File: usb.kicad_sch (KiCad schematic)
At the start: 4 parts, among them J2 SHOU HAN TYPE-C 16PIN 2MD(073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

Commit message: #1 Use new central library KiCad-Lib
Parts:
- J2: footprint Project_Library:SHOU HAN TYPE-C 16PIN 2MD(073) (C2765186) -> #Connector:SHOU HAN TYPE-C 16PIN 2MD(073); symbol Project_Library:SHOU HAN TYPE-C 16PIN 2MD(073) (C2765186) -> #Connector:SHOU HAN TYPE-C 16PIN 2MD(073)
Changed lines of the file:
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@@
     (effects (font (size 1 1)) (justify right))
   )
-  (symbol (lib_id "Project_Library:SHOU HAN TYPE-C 16PIN 2MD(073) (C2765186)") (at 117.475 50.165 0) (mirror y) (unit 1)
+  (symbol (lib_id "#Connector:SHOU HAN TYPE-C 16PIN 2MD(073)") (at 117.475 50.165 0) (mirror y) (unit 1)
     (in_bom yes) (on_board yes) (dnp no)
     (property "Reference" "J2" (at 128.905 48.895 0)
@@
       (effects (font (size 1.27 1.27)) (justify right))
     )
-    (property "Footprint" "Project_Library:SHOU HAN TYPE-C 16PIN 2MD(073) (C2765186)" (at 116.967 82.677 0)
+    (property "Footprint" "#Connector:SHOU HAN TYPE-C 16PIN 2MD(073)" (at 116.967 82.677 0)
       (effects (font (size 1.27 1.27)) hide)
     )
-    (property "Datasheet" "https://datasheet.lcsc.com/lcsc/2111231930_SHOU-HAN-TYPE-C-16PIN-2MD-073_C2765186.pdf" (at 118.999 80.391 0)
+    (property "Datasheet" "${KIPRJMOD}/KiCad-Lib/#Connector.doc/SHOU HAN TYPE-C 16PIN 2MD(073).pdf" (at 118.999 80.391 0)
       (effects (font (size 1.27 1.27)) hide)
     )
@@
       (effects (font (size 1.27 1.27)) hide)
     )
-    (property "JLCPCB Part #" "C2765186" (at 117.475 85.725 0)
+    (property "JLCPCB Part #" "C2765186" (at 117.475 85.725 0) (show_name)
       (effects (font (size 1.27 1.27)) hide)
     )
-    (property "isBasicPart" "NO" (at 117.475 95.885 0)
+    (property "isBasicPart" "NO" (at 117.475 95.885 0) (show_name)
       (effects (font (size 1.27 1.27)) hide)
     )

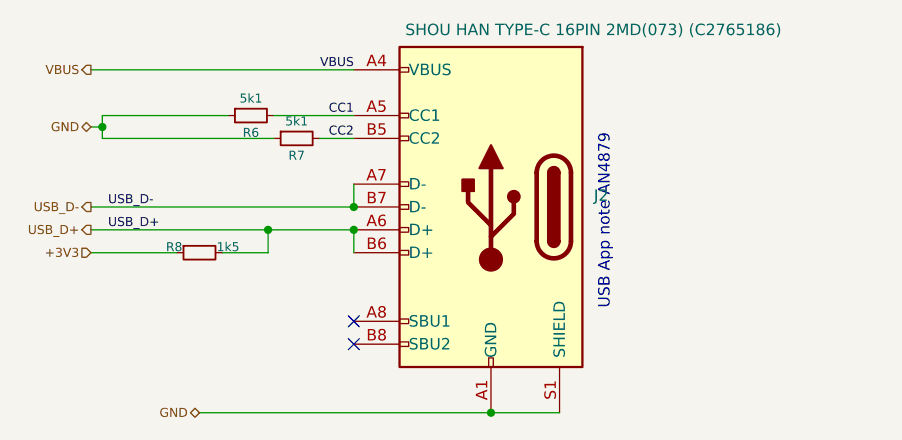
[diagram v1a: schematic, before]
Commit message: WIP
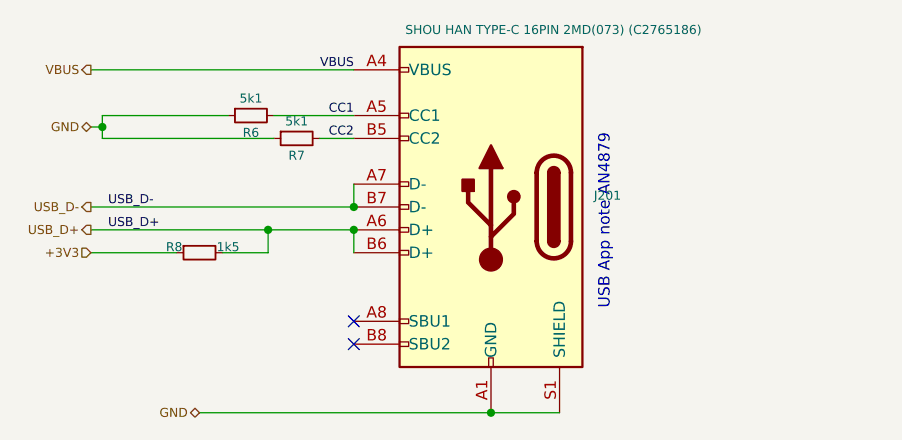
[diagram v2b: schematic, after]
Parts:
- renumbered J2 to J201
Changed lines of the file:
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@@
   (symbol (lib_id "#Connector:SHOU HAN TYPE-C 16PIN 2MD(073)") (at 117.475 50.165 0) (mirror y) (unit 1)
     (in_bom yes) (on_board yes) (dnp no)
-    (property "Reference" "J2" (at 128.905 48.895 0)
-      (effects (font (size 1.27 1.27)) (justify right))
+    (property "Reference" "J201" (at 128.905 48.895 0)
+      (effects (font (size 1 1)) (justify right))
     )
     (property "Value" "SHOU HAN TYPE-C 16PIN 2MD(073) (C2765186)" (at 107.95 30.48 0)
-      (effects (font (size 1.27 1.27)) (justify right))
+      (effects (font (size 1 1)) (justify right))
     )
     (property "Footprint" "#Connector:SHOU HAN TYPE-C 16PIN 2MD(073)" (at 116.967 82.677 0)
@@
       (project "stm32f4_uno"
         (path "/e63e39d7-6ac0-4ffd-8aa3-1841a4541b55/7fb4eaf4-74c6-419d-8578-6cd0a966ea13"
-          (reference "J2") (unit 1)
+          (reference "J201") (unit 1)
         )
       )
@@
         )
         (path "/e63e39d7-6ac0-4ffd-8aa3-1841a4541b55/7fb4eaf4-74c6-419d-8578-6cd0a966ea13"
-          (reference "R401") (unit 1)
+          (reference "R201") (unit 1)
         )
       )
@@
         )
         (path "/e63e39d7-6ac0-4ffd-8aa3-1841a4541b55/7fb4eaf4-74c6-419d-8578-6cd0a966ea13"
-          (reference "R402") (unit 1)
+          (reference "R202") (unit 1)
         )
       )
@@
         )
         (path "/e63e39d7-6ac0-4ffd-8aa3-1841a4541b55/7fb4eaf4-74c6-419d-8578-6cd0a966ea13"
-          (reference "R403") (unit 1)
-        )
-      )
+          (reference "R203") (unit 1)
+        )
+      )
